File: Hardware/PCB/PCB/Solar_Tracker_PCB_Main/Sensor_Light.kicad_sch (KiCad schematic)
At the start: 4 parts, among them IC2 OPT3001DNPRQ1

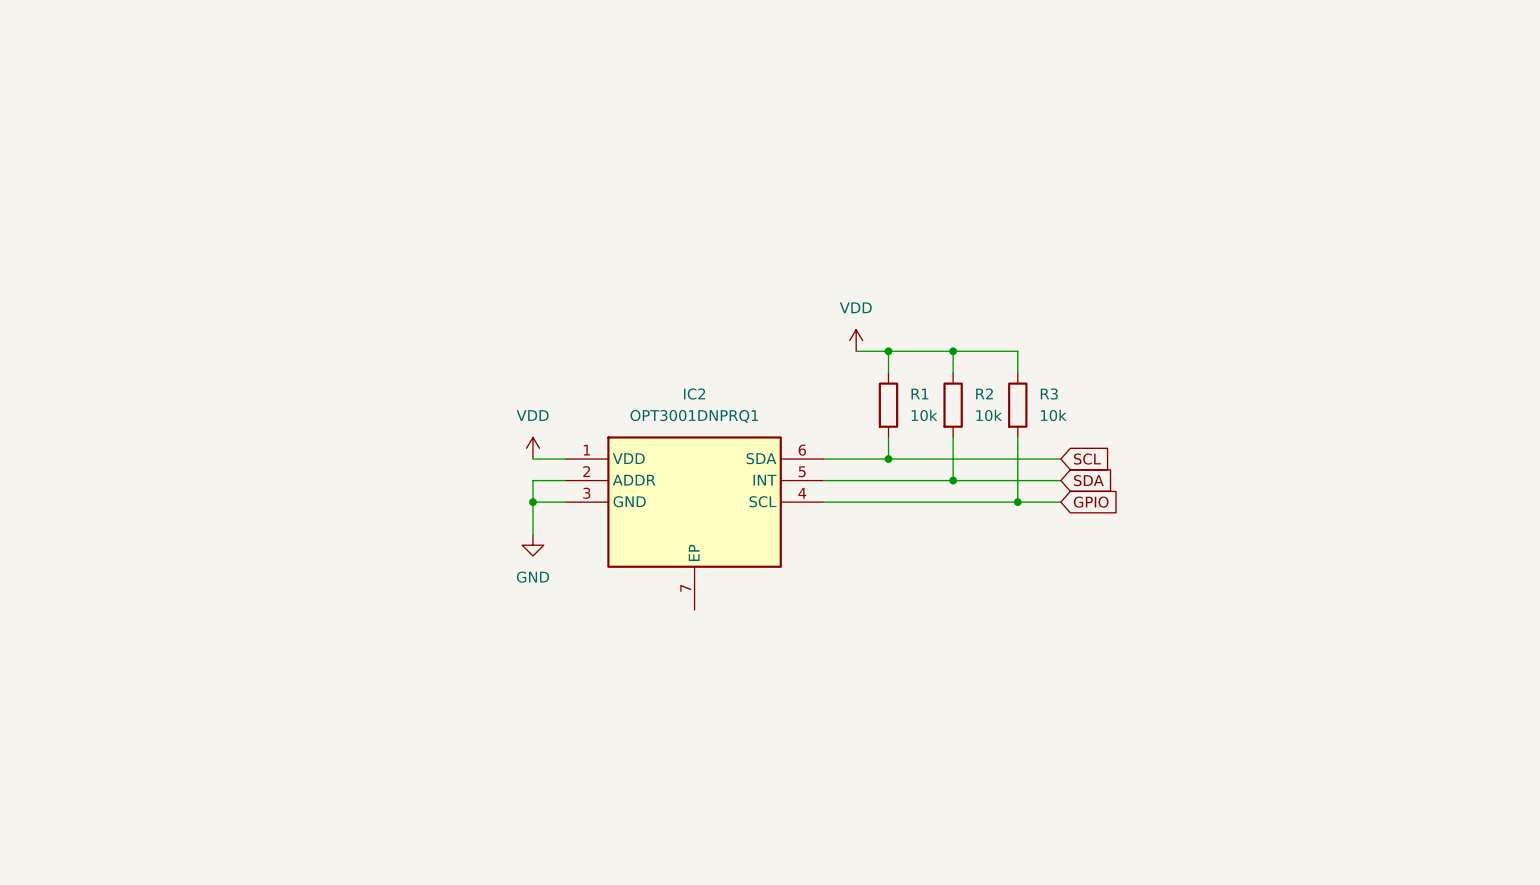
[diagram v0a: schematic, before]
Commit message: pcb
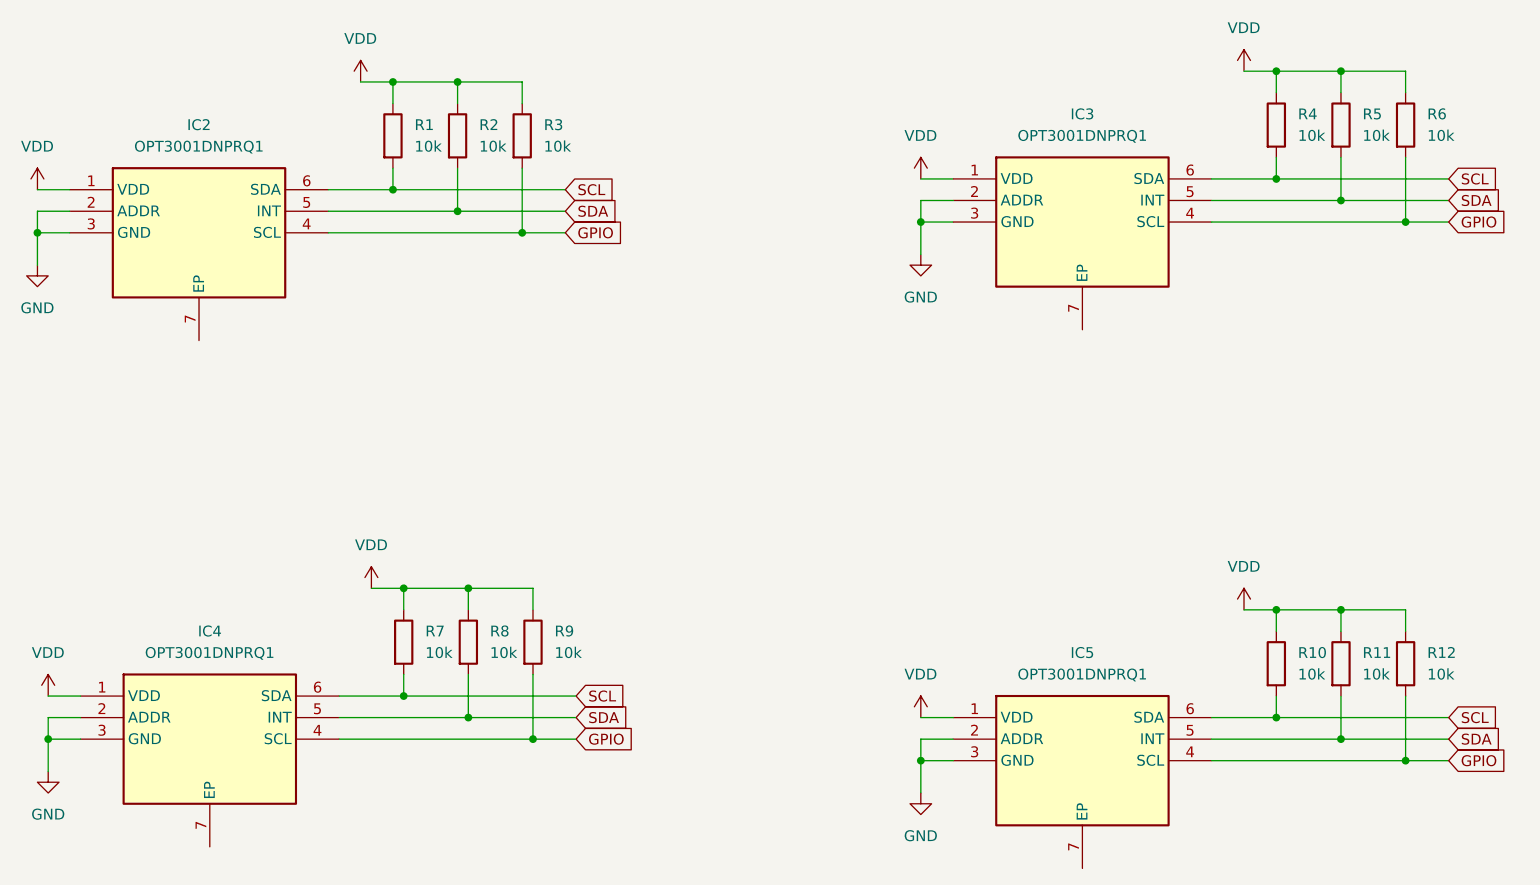
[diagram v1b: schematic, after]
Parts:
- added IC3, IC4, IC5: OPT3001DNPRQ1, OPT3001DNDPRQ1:SON65P200X200X65-7N-D, symbol OPT3001DNPRQ1:OPT3001DNPRQ1
- added R10, R11, R12, R4, R5, R6, R7, R8, R9: 10k, symbol Device:R
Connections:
- net GND: now also IC3.2 (ADDR), IC3.3 (GND), IC4.2 (ADDR), IC4.3 (GND), IC5.2 (ADDR), IC5.3 (GND)
- net GPIO: now also IC3.4 (SCL), IC4.4 (SCL), IC5.4 (SCL), R12.2, R6.2, R9.2
- net SCL: now also IC3.6 (SDA), IC4.6 (SDA), IC5.6 (SDA), R10.2, R4.2, R7.2
- net SDA: now also IC3.5 (INT), IC4.5 (INT), IC5.5 (INT), R11.2, R5.2, R8.2
- net VDD: now also IC3.1 (VDD), IC4.1 (VDD), IC5.1 (VDD), R10.1, R11.1, R12.1, R4.1, R5.1, R6.1, R7.1, R8.1, R9.1
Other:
- moved on the sheet: IC2, R1, R2, R3
